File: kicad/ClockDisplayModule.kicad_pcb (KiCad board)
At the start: 2 copper layers, 91.4 x 58.4 mm, 45 parts, among them IC101 ATMEGA8-P, P101 CONN_02X03, P102 CONN_01X05, P201 CONN_01X06, P202 CONN_01X07, P203 CONN_01X06, P204 CONN_01X07, Q201 BC856BS, Q202 BC856BS, Q203 BC856BS, U201 SN74LS138, U202 74HC4511

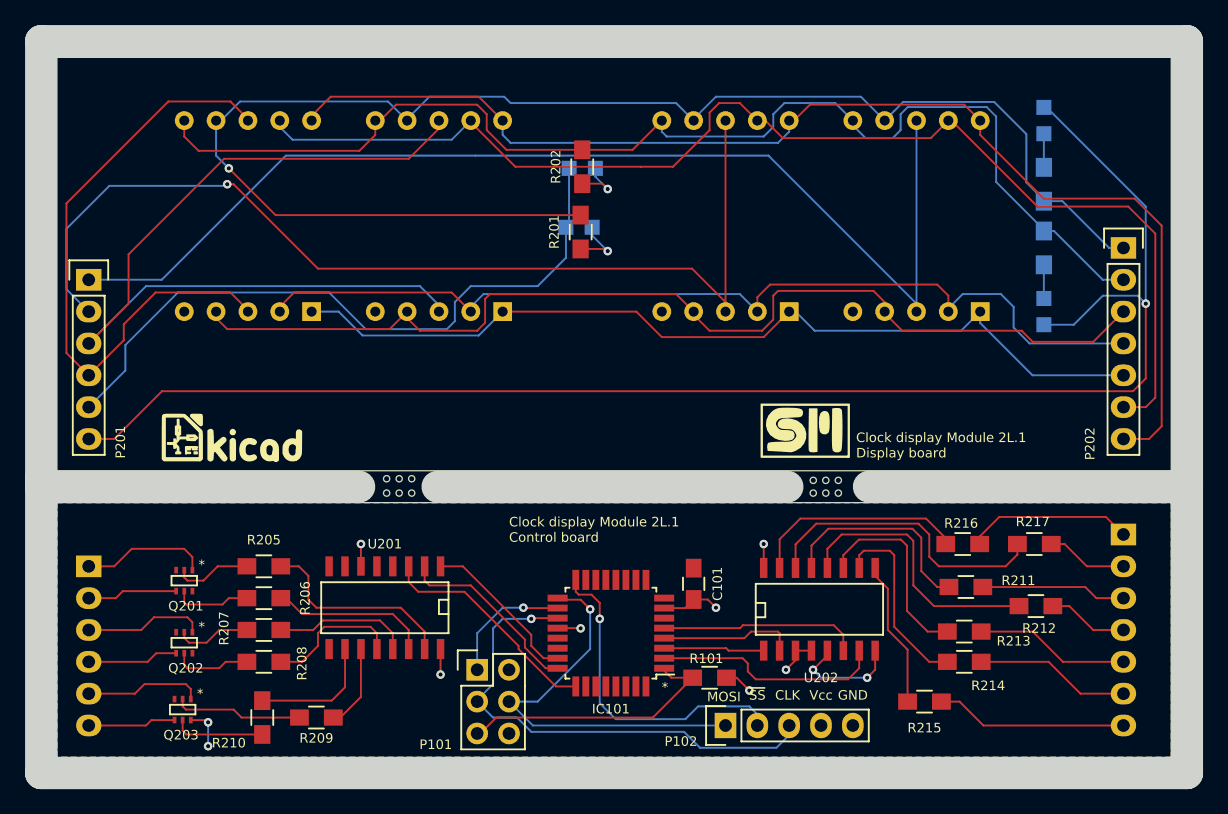
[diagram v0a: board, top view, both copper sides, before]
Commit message: More refinements and updates to logos
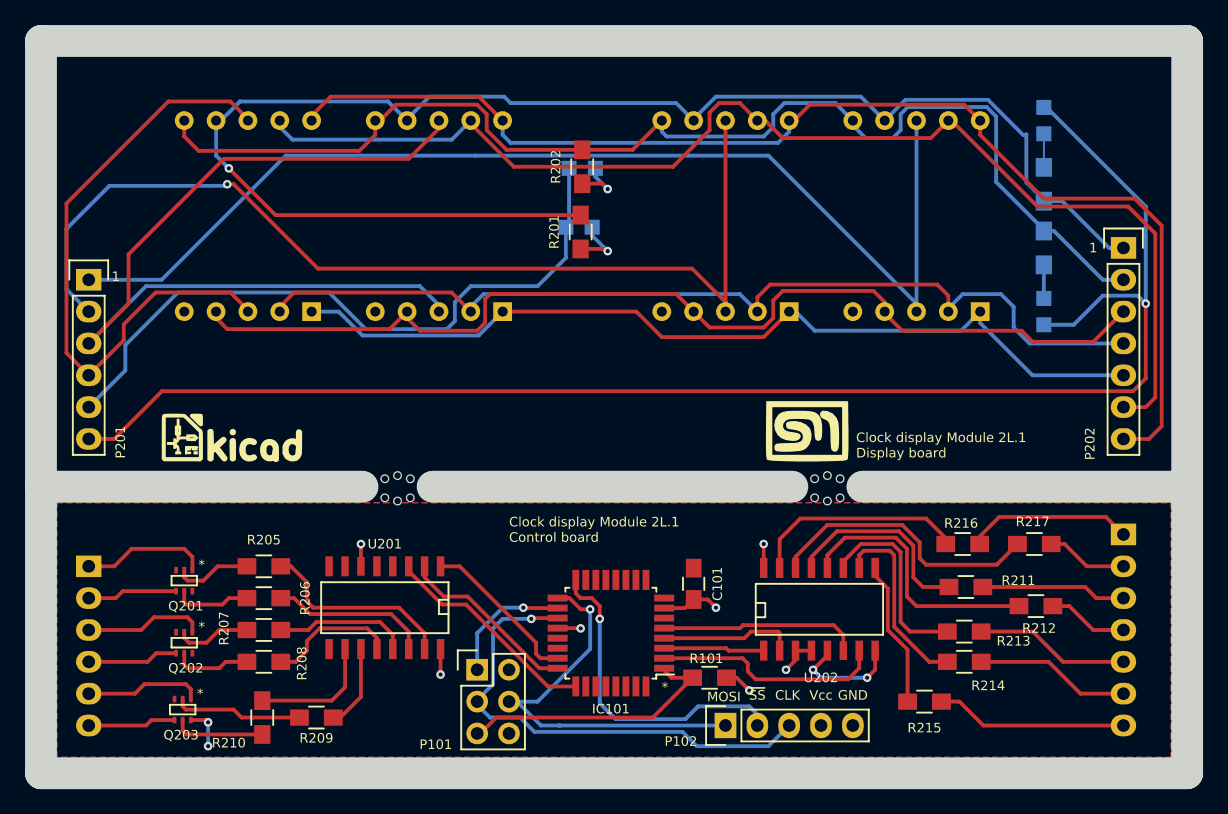
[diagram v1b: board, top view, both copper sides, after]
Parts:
- removed the G*** at (176.5, 73.0)
- removed MouseBite (x4): VAL**, ClockFootprints:MouseBite-npth
- added G***: LOGO, ClockFootprints:myLogo_basic_50, F.Cu at (176.7, 73.0)
- added REF**: MouseBite, ClockFootprints:MouseBite, F.Cu at (143.0, 78.4)
- added REF**: MouseBite, ClockFootprints:MouseBite, F.Cu at (177.3, 78.4)
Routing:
- net Net-(R217-Pad2): track 24.0 -> 22.5 mm
- net Net-(R211-Pad2): track 17.2 -> 16.5 mm
- net A2: track 18.2 -> 17.5 mm
- net A1: track 15.0 -> 14.5 mm
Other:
- outline, holes or cut-outs redrawn
- net class Default: clearance 0.254 -> 0.1524
- rule trace_clearance: 0.254 -> 0.1524
- board text added: "1"
